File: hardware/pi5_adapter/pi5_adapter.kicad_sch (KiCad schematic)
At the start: 15 parts, among them J1 GPIO, J2 GPIO, J3 Conn_01x03_MountingPin, J4 Conn_01x02_Pin, U1 CAT24C256, U2 TPS27081ADDCR

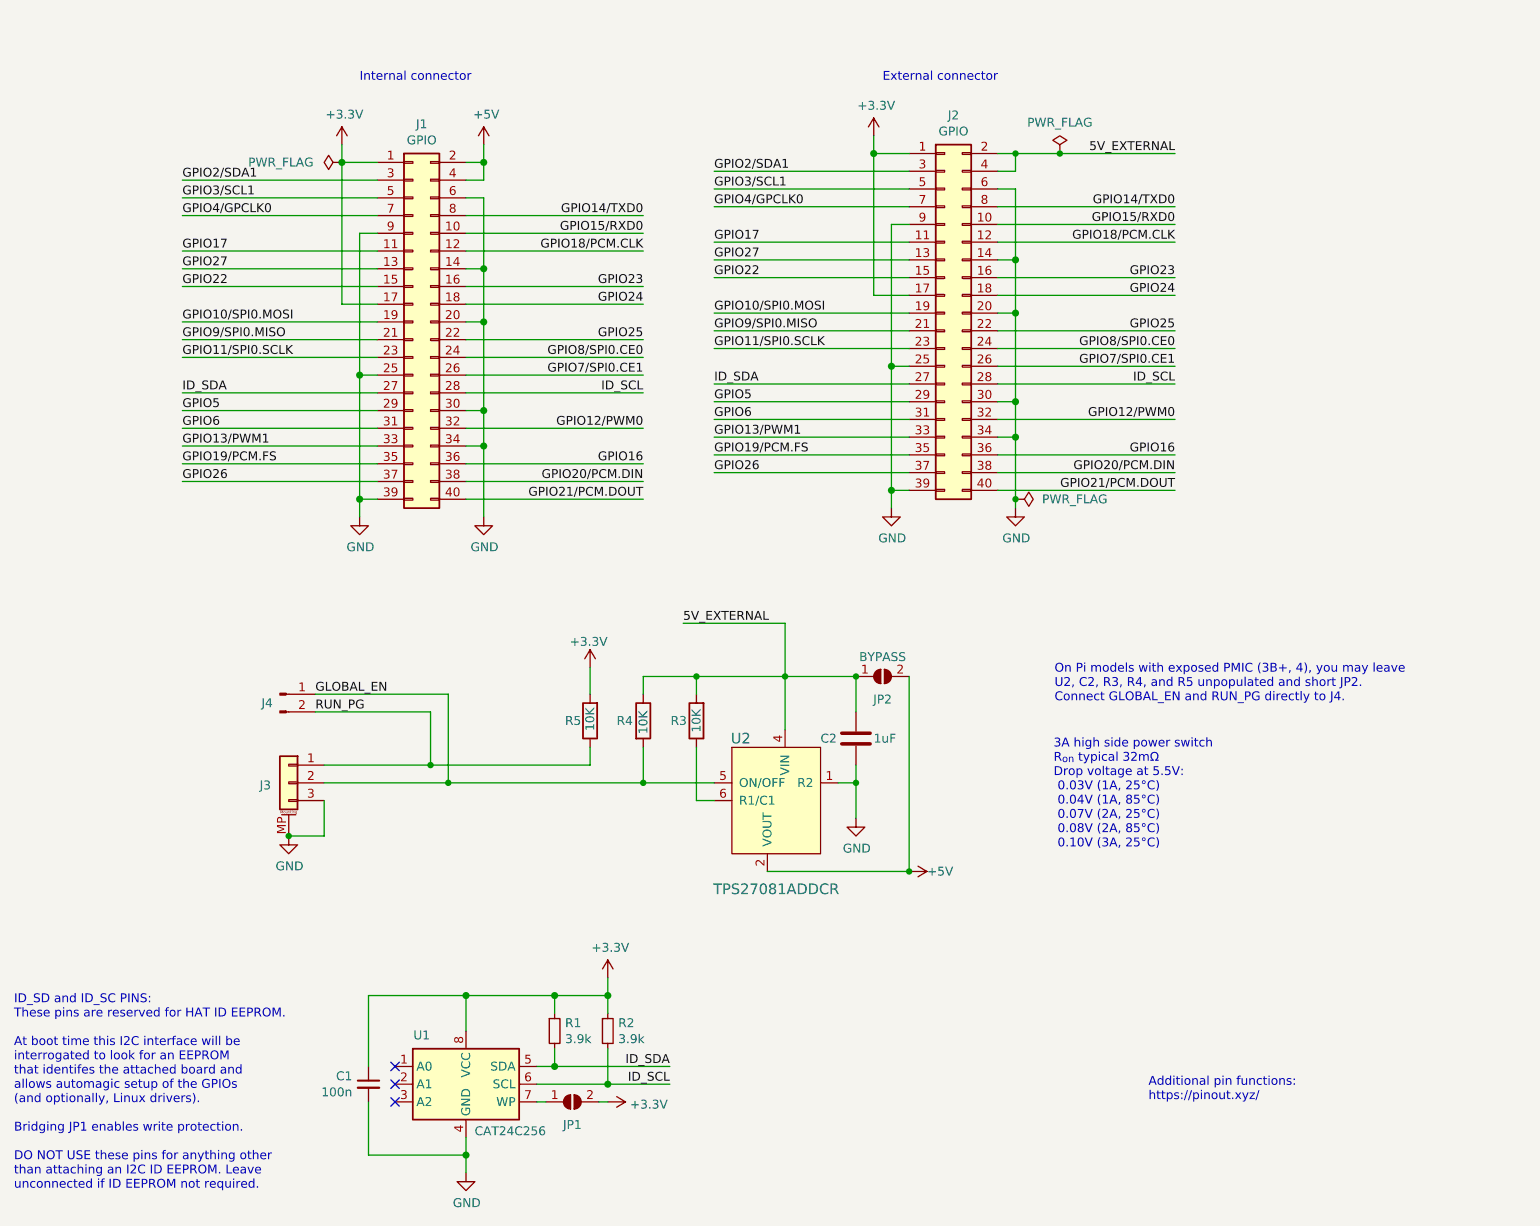
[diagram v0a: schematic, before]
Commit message: pi5_adapter: add 10-pin board to board connector
Problem: the JST jumpers for power are lame.

Add a board to board connector.
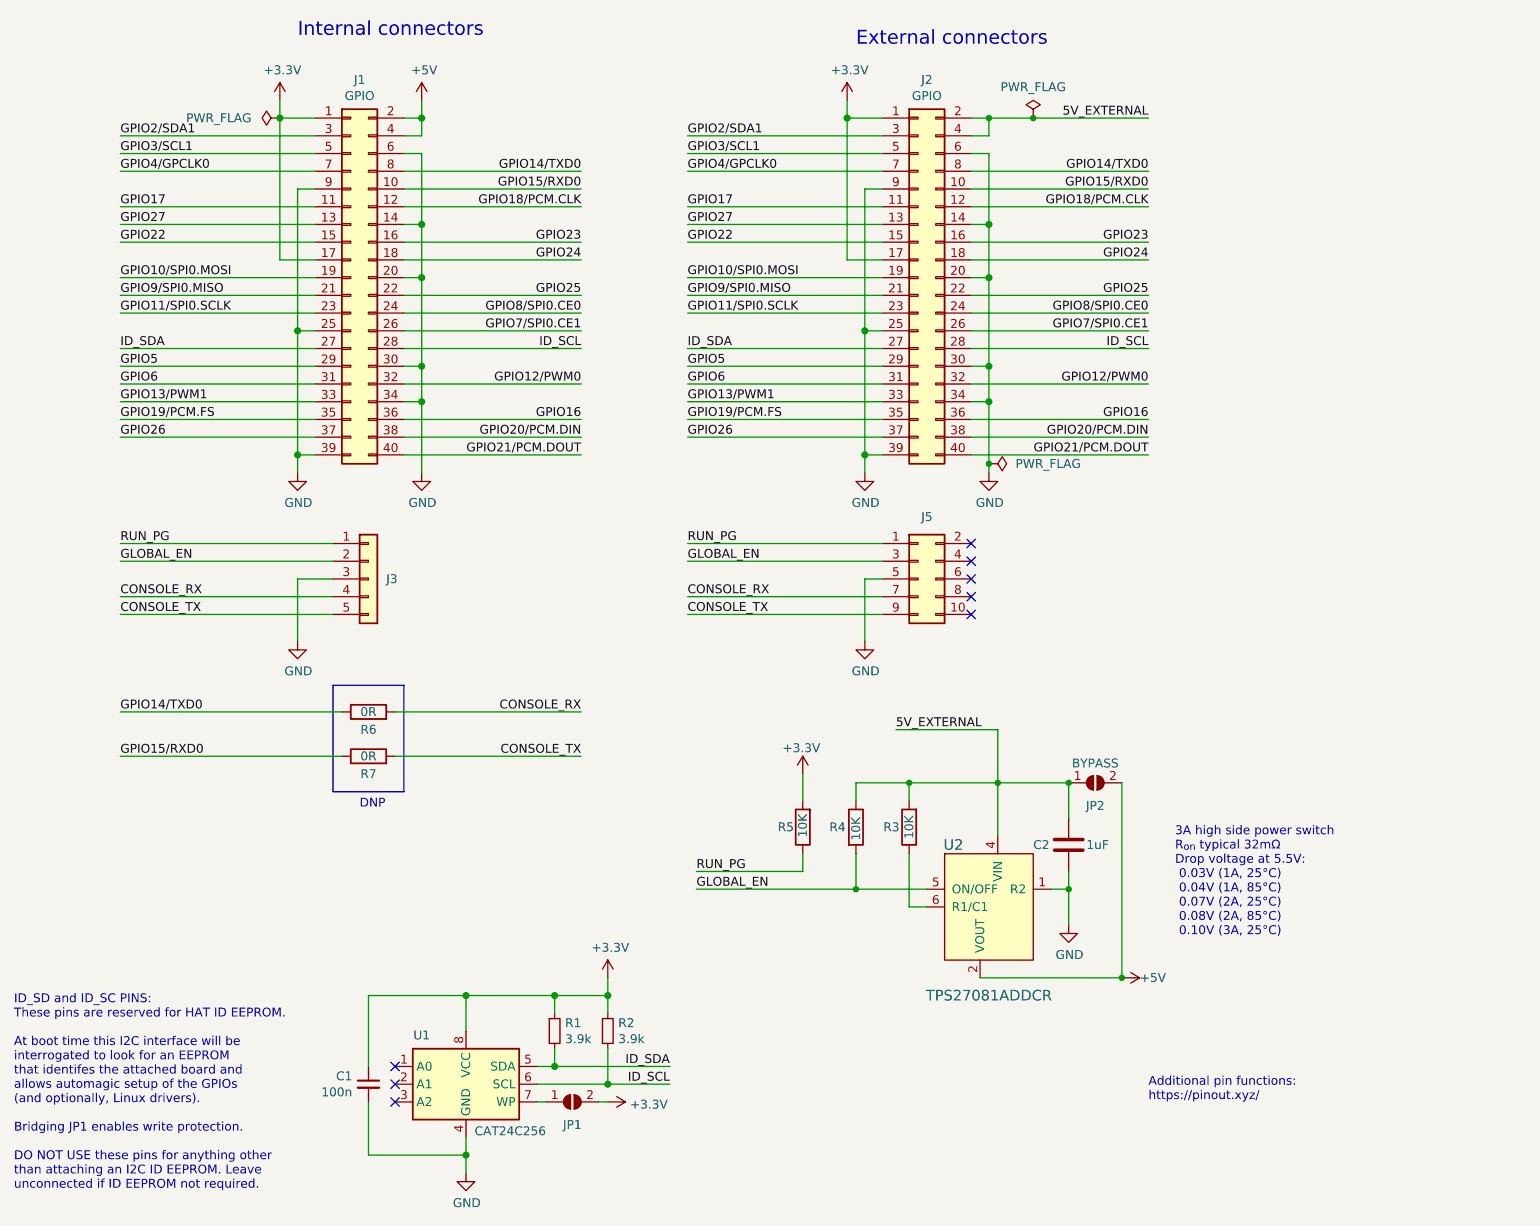
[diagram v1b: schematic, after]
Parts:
- removed J3: Conn_01x03_MountingPin, Connector_JST:JST_SH_BM03B-SRSS-TB_1x03-1MP_P1.00mm_Vertical, symbol Connector_Generic_MountingPin:Conn_01x03_MountingPin
- removed J4: Conn_01x02_Pin, Connector_Wire:SolderWire-0.25sqmm_1x02_P4.2mm_D0.65mm_OD1.7mm, symbol Connector:Conn_01x02_Pin
- added J3: Conn_01x05, lib:PinSocket_1x05_P2.54mm_Vertical, symbol Connector_Generic:Conn_01x05
- added J5: Conn_02x05_Odd_Even, Connector_PinSocket_2.54mm:PinSocket_2x05_P2.54mm_Vertical, symbol Connector_Generic:Conn_02x05_Odd_Even
- added R6, R7: 0R, Resistor_SMD:R_0603_1608Metric, symbol Device:R
- C1: footprint Connector_PinHeader_2.54mm:PinHeader_1x02_P2.54mm_Vertical -> Capacitor_SMD:C_0603_1608Metric
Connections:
- net GLOBAL_EN: now also J3.2 (Pin_2), J5.3 (Pin_3)
- net GND: now also J3.3 (Pin_3), J5.5 (Pin_5)
- net GPIO14/TXD0: now also R6.1
- net GPIO15/RXD0: now also R7.1
- net RUN_PG: now also J3.1 (Pin_1), J5.1 (Pin_1)
- new net CONSOLE_RX: J3.4 (Pin_4), J5.7 (Pin_7), R6.2
- new net CONSOLE_TX: J3.5 (Pin_5), J5.9 (Pin_9), R7.2
- no-connect marks 3 -> 8
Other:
- note added: "DNP"
- note added: "External connectors"
- note added: "Internal connectors"
- note removed: "External connector"
- note removed: "Internal connector"
- note removed: "On Pi models with exposed PMIC (3B+, 4), you may leave U2, C2, R3, R4, and R5 unpopulated and short JP2. Connect GLOBAL_EN and RUN_PG directly to J4."
- moved on the sheet: C2, J1, J2, JP2, R3, R4, R5, U2
